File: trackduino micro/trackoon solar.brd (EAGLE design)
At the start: 57.2 x 19.1 mm, 53 parts, among them IC1 MCP73871, IC2 74AHC1G125DBV, SW1 SPST_TACT-KMR2, U1 ATMEGA168MLF, Y1 16MHZ

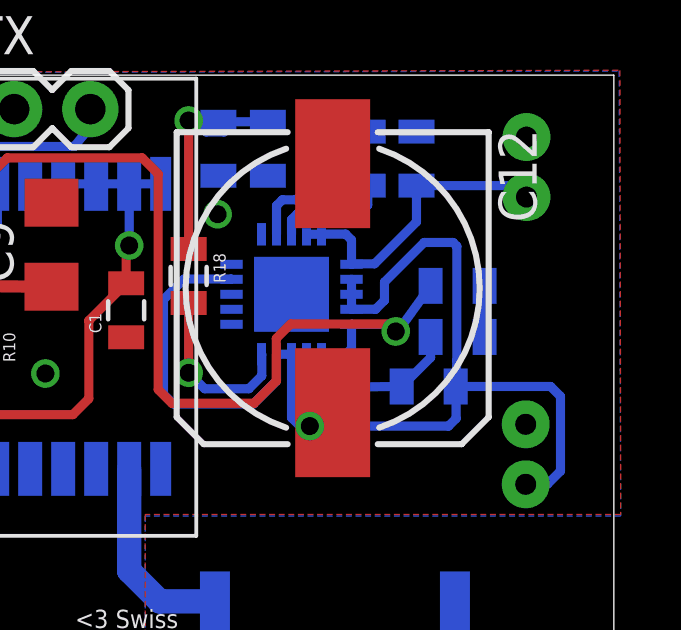
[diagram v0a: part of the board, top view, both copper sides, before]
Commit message: stuff
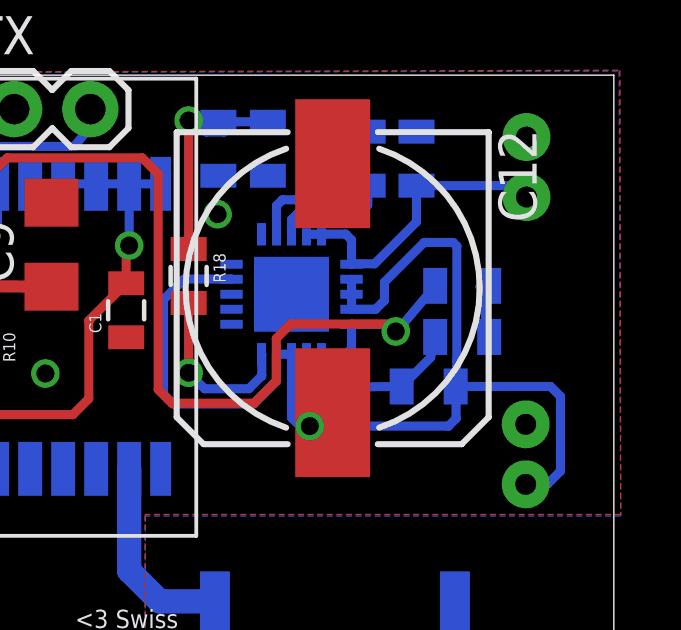
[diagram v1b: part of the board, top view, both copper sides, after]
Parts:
- moved C10 0.15 mm to (61.0, 23.9)
- moved R11 0.15 mm to (61.0, 22.1)
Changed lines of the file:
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@@
 </element>
 <element name="IC1" library="adafruit" package="QFN20" value="MCP73871" x="55.2704" y="23.5712" rot="MR90"/>
-<element name="R11" library="SparkFun-Resistors" package="0805" value="100k" x="60.8076" y="22.1488" rot="MR0"/>
+<element name="R11" library="SparkFun-Resistors" package="0805" value="100k" x="60.96" y="22.1488" rot="MR0"/>
 <element name="R12" library="SparkFun-Resistors" package="0805" value="270k" x="59.8424" y="20.4978" rot="MR180"/>
 <element name="R16" library="SparkFun-Resistors" package="0805" value="2k" x="57.8104" y="28.0924" rot="MR270"/>
 <element name="R17" library="SparkFun-Resistors" package="0805" value="100k" x="56.1594" y="28.1432" rot="MR270"/>
-<element name="C10" library="SparkFun-Capacitors" package="0805" value="10uf" x="60.8076" y="23.8506" rot="MR180"/>
+<element name="C10" library="SparkFun-Capacitors" package="0805" value="10uf" x="60.96" y="23.8506" rot="MR180"/>
 <element name="JP2" library="SparkFun-Connectors" package="JST-2-PTH-VERT" value="M02JST-PTH-VERT" x="63.6524" y="27.813" rot="MR90"/>
 <element name="C11" library="SparkFun-Capacitors" package="0805" value="10uf" x="59.436" y="28.0924" rot="MR90"/>
@@
 <contactref element="JP3" pad="2"/>
 <contactref element="C12" pad="-"/>
-<wire x1="61.7076" y1="22.1488" x2="61.5552" y2="23.8252" width="0.3048" layer="16"/>
-<wire x1="61.5552" y1="23.8252" x2="61.7076" y2="23.8506" width="0.3048" layer="16"/>
+<wire x1="61.86" y1="22.1488" x2="61.5552" y2="23.8252" width="0.3048" layer="16"/>
+<wire x1="61.5552" y1="23.8252" x2="61.86" y2="23.8506" width="0.3048" layer="16"/>
 <via x="52.8066" y="26.2382" extent="1-16" drill="0.6"/>
 <via x="47.0662" y="20.9296" extent="1-16" drill="0.6"/>
@@
 <wire x1="57.2704" y1="22.5712" x2="58.6282" y2="22.5712" width="0.3048" layer="16"/>
 <wire x1="58.6282" y1="22.5712" x2="58.7447" y2="22.3321" width="0.3048" layer="16"/>
-<wire x1="58.9987" y1="22.5861" x2="59.9076" y2="23.8506" width="0.3048" layer="16"/>
+<wire x1="58.9987" y1="22.5861" x2="60.06" y2="23.8506" width="0.3048" layer="16"/>
 <wire x1="43.053" y1="25.6396" x2="43.053" y2="26.7208" width="0.3048" layer="1"/>
 <wire x1="43.053" y1="26.7208" x2="43.6626" y2="27.3304" width="0.3048" layer="1"/>
@@
 <wire x1="55.7704" y1="20.7852" x2="56.0832" y2="20.4724" width="0.3048" layer="16"/>
 <wire x1="56.0832" y1="20.4724" x2="58.9424" y2="20.4978" width="0.3048" layer="16"/>
-<wire x1="59.9076" y1="22.1488" x2="59.9076" y2="21.463" width="0.3048" layer="16"/>
+<wire x1="60.06" y1="22.1488" x2="59.9076" y2="21.463" width="0.3048" layer="16"/>
 <wire x1="59.9076" y1="21.463" x2="58.9424" y2="20.4978" width="0.3048" layer="16"/>
 </signal>
